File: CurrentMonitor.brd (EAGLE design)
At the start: 84 x 67.6 mm, 80 parts, among them IC1 MEGA8-AI, IC2 INA138, IC3 INA138, IC4 LF33CV, J1 AVR_SPI_PRG_6OFFSET_PADS, Q1 10MHz, Q2 IRLZ34N, Q3 IRLZ34N, Q4 IRLZ34N, Q6 BC847, Q7 IRF9530, Q8 IRF9530, Q9 BC847, X1 MSTBA2, X2 MSTBA2, X3 MSTBA2, X5 MSTBA2

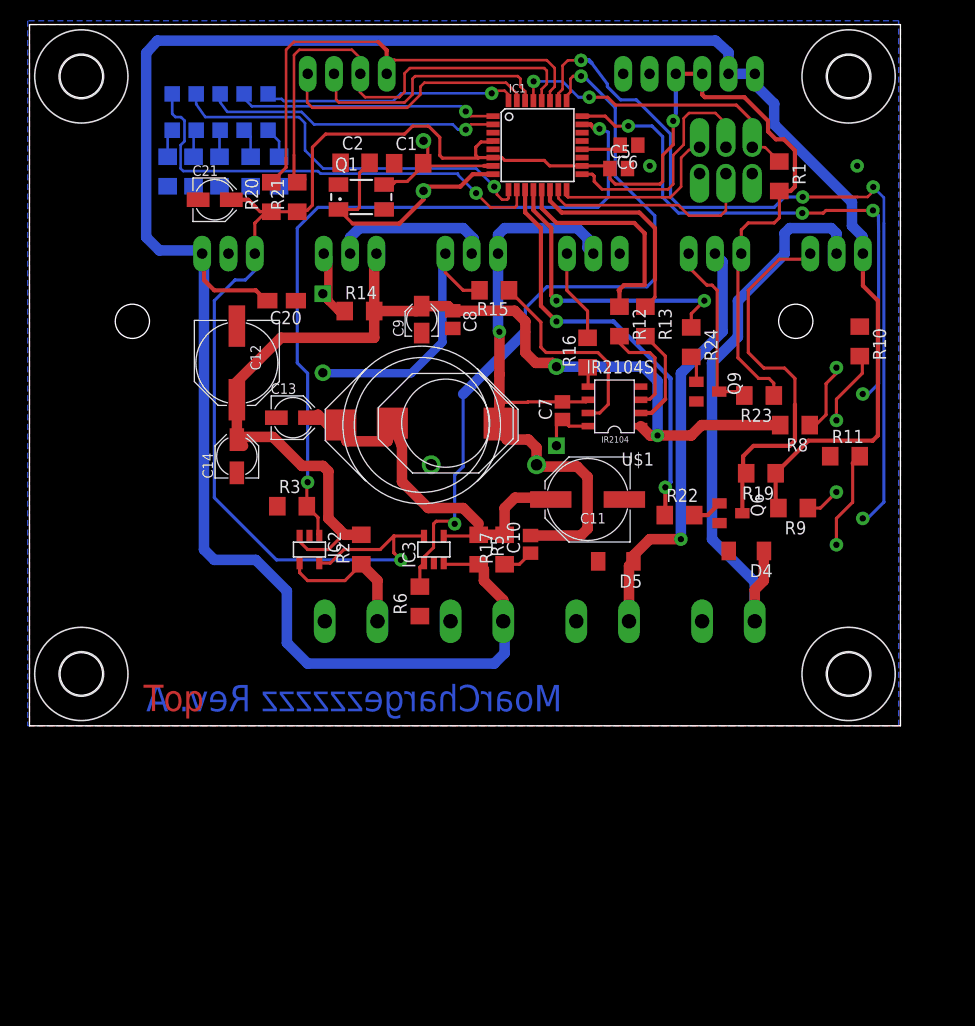
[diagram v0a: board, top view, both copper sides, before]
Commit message: Few fixes (forgot to commit, forgot what I have changed) ;)
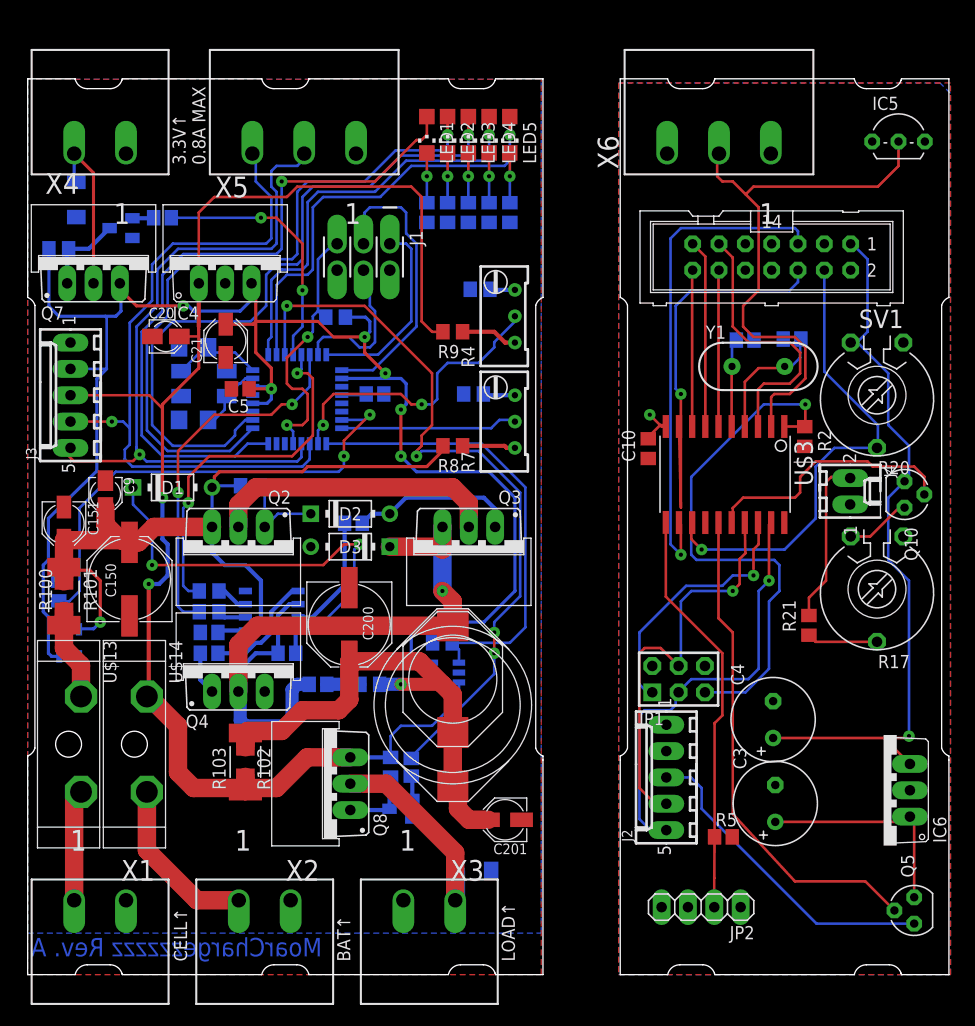
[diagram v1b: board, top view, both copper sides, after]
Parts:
- removed C13, C14: 1µ, rcl:PANASONIC_B
- removed U$4, U$5: (no value), holes:4,1
- added C150, C200: 150µ/25V, rcl:PANASONIC_F
- added C151, C201: 1µ/25V, rcl:PANASONIC_B
- added C202: 100n, resistor:C0805
- added C3, C4: (no value), rcl:E3,5-8
- added IC5: DS18S20, 1wire:TO92-
- added IC6: 7805TV, linear:TO220V
- added J2, J3: 22-27-2051-05, con-molex:6410-05
- added J4: 22-27-2021-02, con-molex:6410-02
- added Q10: BS170, transistor-small-signal:SOT54E
- added R100, R102: 0.1, resistor:R1206
- added R101, R103: 0.005, resistor:R2512
- added R200: 200, rcl:R0805
- added SV1: (no value), con-ml:ML14
- added U$10, U$11, U$12, U$8, U$9: (no value), FischerV5583G:PR5/15-M3
- added U$13, U$14: LITTLEFUSE-178.6164, PudenzCarFuseFLR:LITTLEFUSE-178-6164
- added U$7: (no value), PhoenixContactBCSeries:BC53,6
- added X4: 231-432/001-000, con-wago_5.0mm:P-231-432/001-000
- added X6: 231-433/001-000, con-wago_5.0mm:P-231-433/001-000
- added Y1: (no value), SparkFun:HC49US
- C10: value 100n -> (none); device resistor:C0805 -> rcl:C0805
- C11, C12: value 100µ -> (none); device rcl:PANASONIC_F -> resistor:C0805
- C20: device rcl:A/3216-18R -> rcl:PANASONIC_A
- D3: device diode:DO41-10 -> gm-diodes:DO41-3
- JP1: value (none) -> AVR-ISP-6VERT; device pinhead:1X06 -> avr-7:AVR-ISP-6
- Q5: value (none) -> BS170; device crystal:HC49/S -> transistor-small-signal:SOT54E
- R1, R10, R11, R12, R13, R18, R19, R23, R25, R26, R27, R28, R3, R6, R8, R9: device rcl:R1206 -> rcl:R0805
- R14: device resistor:R1206 -> rcl:R0805
- R15, R16: device resistor:R1206 -> resistor:R0805
- R17: value 200 -> (none); device resistor:R1206 -> pot:PT-10
- R2: value 0.1 -> (none); device resistor:R1206 -> rcl:R0805
- R20: value 10k -> (none); device rcl:R1206 -> pot:PT-10
- R21: value 10k -> (none); device rcl:R1206 -> rcl:R0805
- R22, R24: device rcl:R1206 -> resistor:R0805
- R4, R7: device rcl:RTRIM64P -> rcl:RTRIM64W
- R5: value 0.1 -> (none); device resistor:R1206 -> resistor:R0805
- U$2: device holes:4,1 -> PhoenixContactBCSeries:BC35,6
- U$3: value (none) -> TINY2313-*S*; device holes:4,1 -> avr-7:SO20L$
- U$6: device heatsink:SK125/84 -> FischerV5583G:PR5/15-M3
- X1, X2, X3: value MSTBA2 -> 231-432/001-000; device con-phoenix-508:MSTBA2 -> con-wago_5.0mm:P-231-432/001-000
- X5: value MSTBA2 -> 231-433/001-000; device con-phoenix-508:MSTBA2 -> con-wago_5.0mm:P-231-433/001-000
- moved JP2 87.3 mm to (65.0, 6.51), flipped to the top, turned to 180 degrees
- moved Q5 86.0 mm to (85.5, 6.19), flipped to the top
- moved U$3 73.0 mm to (67.3, 48.2), turned to 180 degrees
- moved Q8 69.3 mm to (28.6, 18.4), flipped to the top, turned to 90 degrees
- moved R23 69.0 mm to (3.00, 70.0), flipped to the bottom
- moved R21 64.4 mm to (75.3, 33.7)
- moved D5 62.7 mm to (4.69, 74.8), flipped to the bottom, turned to 270 degrees
- moved R20 61.5 mm to (81.9, 55.9), turned to 180 degrees
- moved X5 61.4 mm to (26.7, 83.2), flipped to the top, turned to 90 degrees
- moved Q7 60.0 mm to (6.35, 69.2), flipped to the top, turned to 0 degrees
- moved U$2 59.5 mm to (57.1, 0.00)
- moved Q9 58.8 mm to (9.00, 72.0), flipped to the bottom
- moved JP1 58.4 mm to (62.8, 28.5), flipped to the top, turned to 0 degrees
- moved R24 52.4 mm to (13.0, 73.0), flipped to the bottom, turned to 0 degrees
- moved R13 50.5 mm to (17.5, 35.0), flipped to the bottom, turned to 180 degrees
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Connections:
- new net +3V3_2: C10.1, IC5.3, J2.2, JP2.1, R2.2, R5.2, U$3.20, X6.L3
- new net +5V_2: C4.+, IC6.3, Q10.D, R20.E, SV1.1
- new net BAT+CON: U$14.P$2, X2.L1
- new net BAT+_2: J2.3, Q5.D
- new net BGEN: Q10.G, U$3.16
- new net DB4: SV1.11, U$3.3
- new net DB5: SV1.12, U$3.6
- new net DB6: SV1.13, U$3.7
- new net DB7: SV1.14, U$3.8
- new net DISPLAYEN: Q5.G, U$3.15
- new net E: SV1.6, U$3.9
- new net FROM_CELL_CON: U$13.P$2, X1.L1
- new net GND_2: C10.2, C11.1, C12.1, C3.-, C4.-, IC5.1, IC6.2, J2.1, J4.1, JP1.6, JP2.4, R20.A, SV1.2, U$3.10, X6.L1
- new net N$15: R17.S, R21.1
- new net N$19: JP2.2, R5.1, U$3.11
- new net N$24: J4.2, R21.2
- new net N$27: JP1.5, R2.1, U$3.1
- new net N$28: Q10.S, R17.E
- new net N$30: C11.2, U$3.4, Y1.2
- new net N$31: C12.2, U$3.5, Y1.1
- new net N$33: C3.+, IC6.1, Q5.S
- new net N$35: U$3.14
- new net N$7: JP1.1, U$3.18
- new net OW: IC5.2, U$3.2, X6.L2
- new net R/W: SV1.5, U$3.12
- new net RS: R20.S, SV1.4, U$3.13
- new net SCL2: J2.5, JP1.3, U$3.19
- new net SDA2: J2.4, JP1.4, U$3.17
- new net V0: SV1.3
- net +3V3: now also J3.2; no longer JP1.3, JP1.4, R20.1, R21.1
- net BAT+: now also J3.3, R102.2, R103.1, U$14.P$1; no longer JP1.5, JP1.6, R5.2, X2.1
- net CELL_TO_CONTROLLER: now also C150.+, C151.+, R100.2, R101.1; no longer C12.+, C14.+, R2.2
- net CONTROLLER_TO_BAT: now also C200.+, C201.+, R102.1, R103.2, R200.2; no longer C11.+, C13.+, R17.2, R5.1
- net FROM_CELL: now also R100.1, R101.2, U$13.P$1; no longer R2.1, X1.1
- net GND: now also C150.-, C151.-, C200.-, C201.-, J3.1, X1.L2, X2.L2, X3.L1, X4.L1, X5.L1; no longer C11.-, C12.-, C13.-, C14.-, JP1.1, JP1.2, X1.2, X2.2, X3.2, X5.2
- net N$16: now also X3.L2; no longer X3.1
- net N$17: now also C202.1, R200.1; no longer C10.1, R17.1
- net N$25: now also X4.L2; no longer X5.1
- net RXD: no longer JP2.3
- net SCL: now also J3.5, X5.L2; no longer JP2.2, R21.2
- net SDA: now also J3.4, X5.L3; no longer JP2.1, R20.2
- net TXD: no longer JP2.4
- net VS: now also C202.2; no longer C10.2
- net XTAL1: no longer Q5.2
- net XTAL2: no longer Q5.1
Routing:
- net BAT+: track 228.2 -> 143.4 mm, vias 0 -> 2
- net +5V_2: track 0.00 -> 70.3 mm, vias 0 -> 1
- net OW: track 0.00 -> 54.6 mm
- net N$27: track 0.00 -> 52.0 mm, vias 0 -> 1
- net ADC3: track 78.0 -> 28.9 mm, vias 3 -> 2
- net DISPLAYEN: track 0.00 -> 48.3 mm
- net R/W: track 0.00 -> 48.1 mm, vias 0 -> 1
- net RS: track 0.00 -> 46.3 mm, vias 0 -> 1
- net LED1: track 24.6 -> 66.5 mm
- net SCL2: track 0.00 -> 41.6 mm, vias 0 -> 1
- net E: track 0.00 -> 41.4 mm, vias 0 -> 1
- net LED2: track 25.8 -> 65.9 mm
- net SDA2: track 0.00 -> 39.8 mm, vias 0 -> 1
- net N$19: track 0.00 -> 39.7 mm
- net LED3: track 28.5 -> 66.5 mm
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- added copper zone on layer 1, net +3V3_2
- added copper zone on layer 16, net GND_2
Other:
- board size 84 x 67.6 mm -> 49.7 x 86.4 mm
- board text added: "3.3V↑ 0.8A MAX"
- board text added: "BAT↑"
- board text added: "CELL↑"
- board text added: "LOAD↑"
- board text added: "Note: Trace Width for High Power Tracks (10A) is 72 mil for 70µm copper with 30°C temp rise at ambient 25°C. This is enough to cover an ambient temperature up to 60°C. Note that if you etch this board on 35µm copper you're limited to about 6A. Silkscreen is not adjusted yet due to prototype status. Check back later :-)"
- board text removed: "Top"
